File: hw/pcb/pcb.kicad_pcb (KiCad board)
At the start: 2 copper layers, 99.1 x 67.3 mm, 67 parts, among them J1 ConnMain, J2 ConnPorts, J3 Conn_01x01_Pin, J4 Conn_01x01_Pin, J5 Conn_01x01_Pin, J6 Conn_01x01_Pin

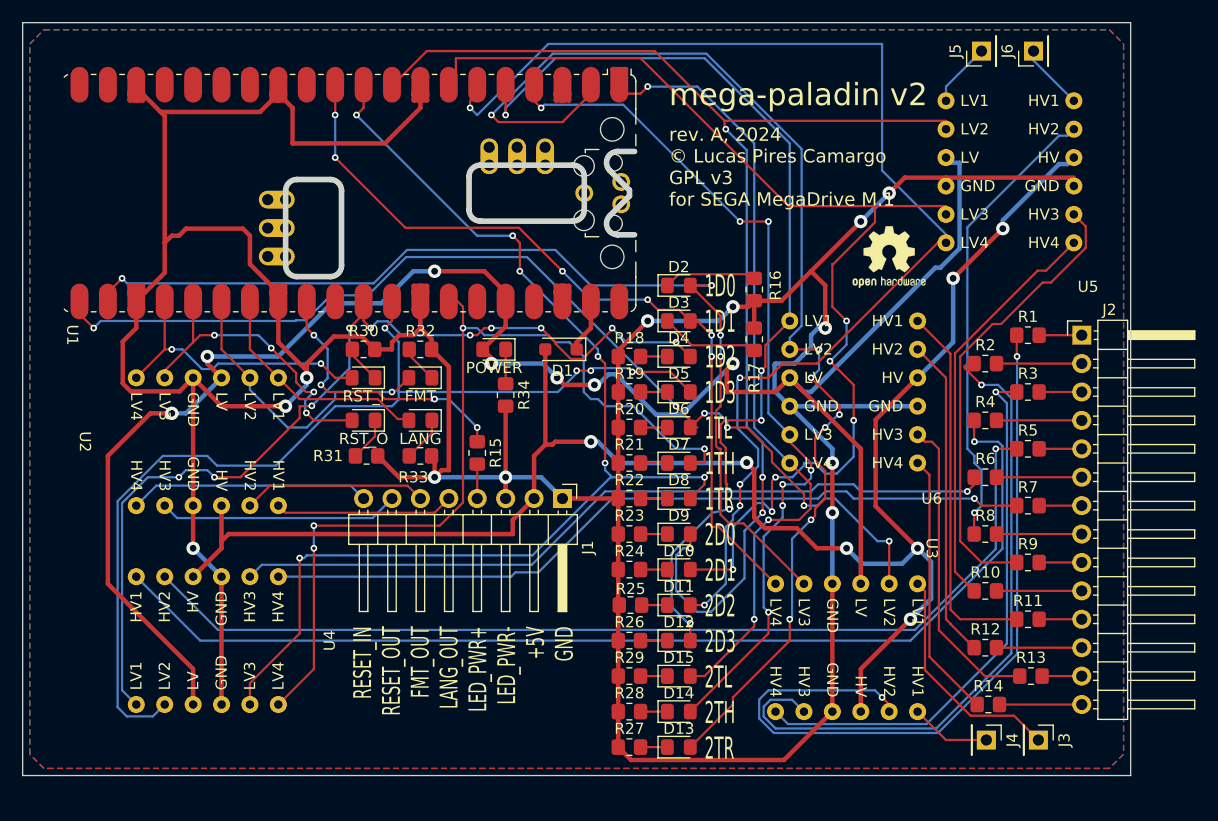
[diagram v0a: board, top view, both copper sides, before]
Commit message: [hw] initial v3 design, updated readme
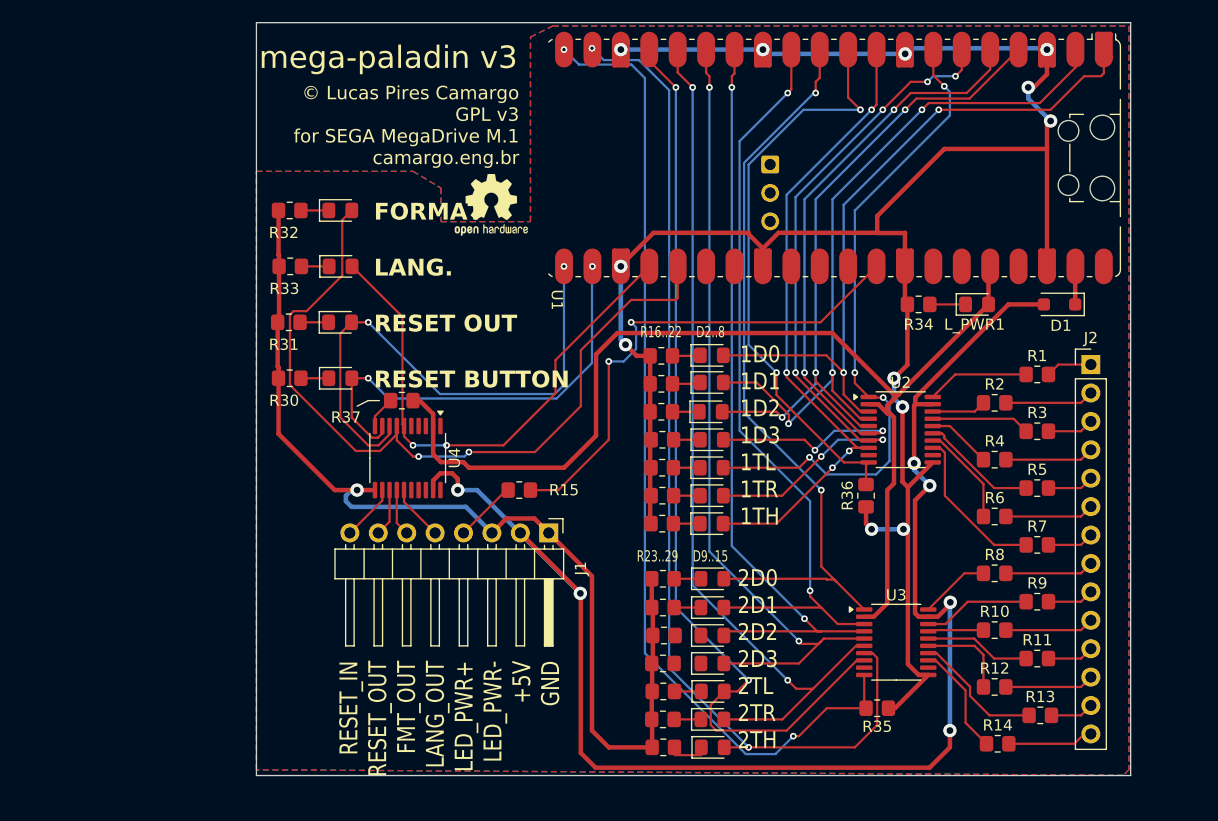
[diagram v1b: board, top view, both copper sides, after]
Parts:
- removed J3, J4, J5, J6: Conn_01x01_Pin, Connector_PinHeader_2.54mm:PinHeader_1x01_P2.54mm_Vertical
- removed U5, U6: ~, footprints:cheap_lvl_shifter_4ch
- added R35: 1K, Resistor_SMD:R_0805_2012Metric_Pad1.20x1.40mm_HandSolder, F.Cu at (114.5, 90.5)
- added R36: 1K, Resistor_SMD:R_0805_2012Metric_Pad1.20x1.40mm_HandSolder, F.Cu at (113.5, 71.5)
- added R37: 1K, Resistor_SMD:R_0805_2012Metric_Pad1.20x1.40mm_HandSolder, F.Cu at (72.0, 63.0)
- J2: footprint Connector_PinHeader_2.54mm:PinHeader_1x14_P2.54mm_Horizontal -> Connector_PinHeader_2.54mm:PinHeader_1x14_P2.54mm_Vertical
- R1, R10, R11, R12, R13, R14, R2, R3, R4, R5, R6, R7, R8, R9: value 10K -> 1K
- U1: footprint Module_RaspberryPi_Pico:RaspberryPi_Pico_W_SMD_MountingHoles_Castellated_HandSolder -> Module:RaspberryPi_Pico_W_SMD_HandSolder
- U2, U3, U4: value ~ -> TXS0108EPW; footprint footprints:cheap_lvl_shifter_4ch -> Package_SO:TSSOP-20_4.4x6.5mm_P0.65mm
- moved U2 73.4 mm to (116.6, 65.6), turned to 0 degrees
- moved D1 44.8 mm to (130.8, 54.4)
- moved U1 43.4 mm to (110.6, 41.3)
- moved L_PWR1 43.4 mm to (123.4, 54.4), turned to 0 degrees
- moved R34 37.8 mm to (118.2, 54.4), turned to 180 degrees
- moved REF** 35.9 mm to (80.0, 45.5)
- moved R33 20.6 mm to (62.0, 51.0), turned to 180 degrees
- moved U4 17.6 mm to (72.5, 68.1), turned to -90 degrees
- moved R32 17.1 mm to (62.0, 46.0), turned to 180 degrees
- moved L_FMT_OUT1 16.6 mm to (66.5, 46.0), turned to 0 degrees
- moved U3 15.9 mm to (116.2, 84.6), turned to 0 degrees
- moved L_LANG_OUT1 15.5 mm to (66.5, 51.0), turned to 0 degrees
- moved R31 13.8 mm to (61.9, 56.0), turned to 180 degrees
- moved R16 10.2 mm to (95.2, 59.0), turned to 0 degrees
- moved R17 9.21 mm to (95.2, 61.5), turned to 0 degrees
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- renumbered FMT to L_FMT_OUT1, LANG to L_LANG_OUT1, POWER to L_PWR1, RST_I to L_R_IN1, RST_O to L_R_OUT1
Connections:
- D13 pad 2: /P2_6_LV -> /P2_4_LV
- D15 pad 2: /P2_4_LV -> /P2_6_LV
- J2 pad 12: /P2_6 -> /P2_5
- J2 pad 13: /P2_5 -> /P2_6
- J2 pad 6: /P1_6 -> /P1_5
- J2 pad 7: /P1_5 -> /P1_6
- R1 pad 1: Net-(U3-HV2) -> Net-(U2-B1)
- R10 pad 1: Net-(U5-HV4) -> Net-(U3-B3)
- R11 pad 1: Net-(U6-HV1) -> Net-(U3-B4)
- R12 pad 1: Net-(U6-HV2) -> Net-(U3-B5)
- R12 pad 2: /P2_6 -> /P2_5
- R13 pad 1: Net-(U6-HV3) -> Net-(U3-B6)
- R13 pad 2: /P2_5 -> /P2_6
- R14 pad 1: Net-(U6-HV4) -> Net-(U3-B7)
- R15 pad 1: Net-(U1-GP22) -> Net-(U1-GPIO27_ADC1)
- R2 pad 1: Net-(U3-HV3) -> Net-(U2-B2)
- R3 pad 1: Net-(U3-HV4) -> Net-(U2-B3)
- R4 pad 1: Net-(U4-HV1) -> Net-(U2-B4)
- R5 pad 1: Net-(U4-HV2) -> Net-(U2-B5)
- R6 pad 1: Net-(U4-HV3) -> Net-(U2-B6)
- R6 pad 2: /P1_6 -> /P1_5
- R7 pad 1: Net-(U4-HV4) -> Net-(U2-B7)
- R7 pad 2: /P1_5 -> /P1_6
- R8 pad 1: Net-(U5-HV2) -> Net-(U3-B1)
- R9 pad 1: Net-(U5-HV3) -> Net-(U3-B2)
- U1 pad 1: /P2_4_LV -> /P1_0_LV
- U1 pad 10: /P1_6_LV -> /P1_OE
- U1 pad 11: /P1_1_LV -> /P2_0_LV
- U1 pad 12: unconnected-(U1-GP9-Pad12) -> /P2_1_LV
- U1 pad 14: unconnected-(U1-GP10-Pad14) -> /P2_2_LV
- U1 pad 15: unconnected-(U1-GP11-Pad15) -> /P2_3_LV
- U1 pad 16: unconnected-(U1-GP12-Pad16) -> /P2_5_LV
- U1 pad 17: unconnected-(U1-GP13-Pad17) -> /P2_4_LV
- U1 pad 19: unconnected-(U1-GP14-Pad19) -> /P2_6_LV
- U1 pad 2: /P2_6_LV -> /P1_1_LV
- U1 pad 20: unconnected-(U1-GP15-Pad20) -> /P2_OE
- U1 pad 21: /P1_4_LV -> /OUT_RESET_LV
- U1 pad 22: /P1_0_LV -> /IN_RESET_LV
- U1 pad 24: /IN_RESET_LV -> /OUT_LANG_LV
- U1 pad 25: /OUT_RESET_LV -> /OUT_FMT_LV
- U1 pad 26: /OUT_FMT_LV -> unconnected-(U1-GPIO20-Pad26)
- U1 pad 27: /OUT_LANG_LV -> unconnected-(U1-GPIO21-Pad27)
- U1 pad 29: Net-(U1-GP22) -> unconnected-(U1-GPIO22-Pad29)
- U1 pad 3: unconnected-(U1-GND-Pad3) -> GND
- U1 pad 31: /P1_2_LV -> unconnected-(U1-GPIO26_ADC0-Pad31)
- U1 pad 32: /P1_3_LV -> Net-(U1-GPIO27_ADC1)
- U1 pad 34: /P1_5_LV -> unconnected-(U1-GPIO28_ADC2-Pad34)
- U1 pad 38: (no net) -> GND
- U1 pad 4: /P2_5_LV -> /P1_2_LV
- U1 pad 5: /P2_3_LV -> /P1_3_LV
- U1 pad 6: /P2_2_LV -> /P1_5_LV
- U1 pad 7: /P2_1_LV -> /P1_4_LV
- U1 pad 9: /P2_0_LV -> /P1_6_LV
- U2 pad 1: /OUT_LANG_LV -> /P1_4_LV
- U2 pad 10: +5V -> /P1_OE
- U2 pad 11: /OUT_FMT -> GND
- U2 pad 12: /OUT_LANG -> unconnected-(U2-B8-Pad12)
- U2 pad 2: /OUT_FMT_LV -> +3V3
- U2 pad 3: +3V3 -> /P1_0_LV
- U2 pad 4: GND -> /P1_1_LV
- U2 pad 5: /OUT_RESET_LV -> /P1_2_LV
- U2 pad 6: /IN_RESET_LV -> /P1_3_LV
- U2 pad 7: /IN_RESET -> /P1_5_LV
- U2 pad 8: /OUT_RESET -> /P1_6_LV
- U2 pad 9: GND -> unconnected-(U2-A8-Pad9)
- U3 pad 1: Net-(J3-Pin_1) -> /P2_0_LV
- U3 pad 10: +5V -> /P2_OE
- U3 pad 11: Net-(U3-HV2) -> GND
- U3 pad 12: Net-(J4-Pin_1) -> unconnected-(U3-B8-Pad12)
- U3 pad 2: /P1_4_LV -> +3V3
- U3 pad 3: +3V3 -> /P2_1_LV
- U3 pad 4: GND -> /P2_2_LV
- U3 pad 5: /P1_0_LV -> /P2_3_LV
- U3 pad 6: /P1_1_LV -> /P2_5_LV
- U3 pad 7: Net-(U3-HV4) -> /P2_6_LV
- U3 pad 8: Net-(U3-HV3) -> /P2_4_LV
- U3 pad 9: GND -> unconnected-(U3-A8-Pad9)
- U4 pad 1: /P1_2_LV -> unconnected-(U4-A1-Pad1)
- U4 pad 10: +5V -> Net-(U4-OE)
- U4 pad 11: Net-(U4-HV2) -> GND
- U4 pad 12: Net-(U4-HV1) -> /IN_RESET
- U4 pad 2: /P1_3_LV -> +3V3
- U4 pad 3: +3V3 -> unconnected-(U4-A2-Pad3)
- U4 pad 4: GND -> unconnected-(U4-A3-Pad4)
- U4 pad 5: /P1_6_LV -> unconnected-(U4-A4-Pad5)
- U4 pad 6: /P1_5_LV -> /OUT_LANG_LV
- U4 pad 7: Net-(U4-HV4) -> /OUT_FMT_LV
- U4 pad 8: Net-(U4-HV3) -> /OUT_RESET_LV
- U4 pad 9: GND -> /IN_RESET_LV
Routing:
- net Net-(U4-HV1): track 97.0 -> 0.00 mm, vias 1 -> 0
- net Net-(U4-HV2): track 90.1 -> 0.00 mm, vias 1 -> 0
- net /P2_OE: track 0.00 -> 87.9 mm, vias 0 -> 2
- net GND: track 361.7 -> 282.5 mm, vias 12 -> 13
- net Net-(U3-HV2): track 69.8 -> 0.00 mm, vias 2 -> 0
- net Net-(U4-HV4): track 69.7 -> 0.00 mm, vias 1 -> 0
- net Net-(U4-HV3): track 69.3 -> 0.00 mm, vias 1 -> 0
- net +3V3: track 165.2 -> 98.7 mm, vias 7 -> 0
- net Net-(U3-HV3): track 59.8 -> 0.00 mm, vias 1 -> 0
- net /P1_OE: track 0.00 -> 52.3 mm, vias 0 -> 2
- net Net-(U3-HV4): track 48.9 -> 0.00 mm, vias 1 -> 0
- net Net-(U1-GPIO27_ADC1): track 0.00 -> 45.3 mm, vias 0 -> 2
- net /P1_6_LV: track 102.4 -> 58.4 mm, vias 7 -> 4
- net /P2_0_LV: track 111.2 -> 67.5 mm, vias 4 -> 2
- net /OUT_FMT_LV: track 27.6 -> 69.8 mm, vias 1 -> 2
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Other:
- board size 99.1 x 67.3 mm -> 78.2 x 67.3 mm
- board text added: "1D0 1D1 1D2 1D3 1TL 1TR 1TH"
- board text added: "2D0 2D1 2D2 2D3 2TL 2TR 2TH"
- board text added: "D2..8"
- board text added: "D9..15"
- board text added: "FORMAT"
- board text added: "LANG."
- board text added: "R16..22"
- board text added: "R23..29"
- board text added: "RESET BUTTON"
- board text added: "RESET OUT"
- board text added: "mega-paladin v3"
- board text added: "© Lucas Pires Camargo GPL v3 for SEGA MegaDrive M.1 camargo.eng.br"
- board text removed: "1D0 1D1 1D2 1D3 1TL 1TH 1TR 2D0 2D1 2D2 2D3 2TL 2TH 2TR"
- board text removed: "TODO: fix level shifter footprint dimensions get the micro usb connector on the board edge, duh!!!!! 10k seems to be too high for input protection, cannot read controllers that way and creates a voltage divider. Change to 1k!"
- board text removed: "mega-paladin v2"
- board text removed: "rev. A, 2024 © Lucas Pires Camargo GPL v3 for SEGA MegaDrive M.1"
